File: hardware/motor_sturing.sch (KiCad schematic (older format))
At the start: 6 parts, among them U1 LTC2351-14, U22 LTC2351-14, U5 MAX6101

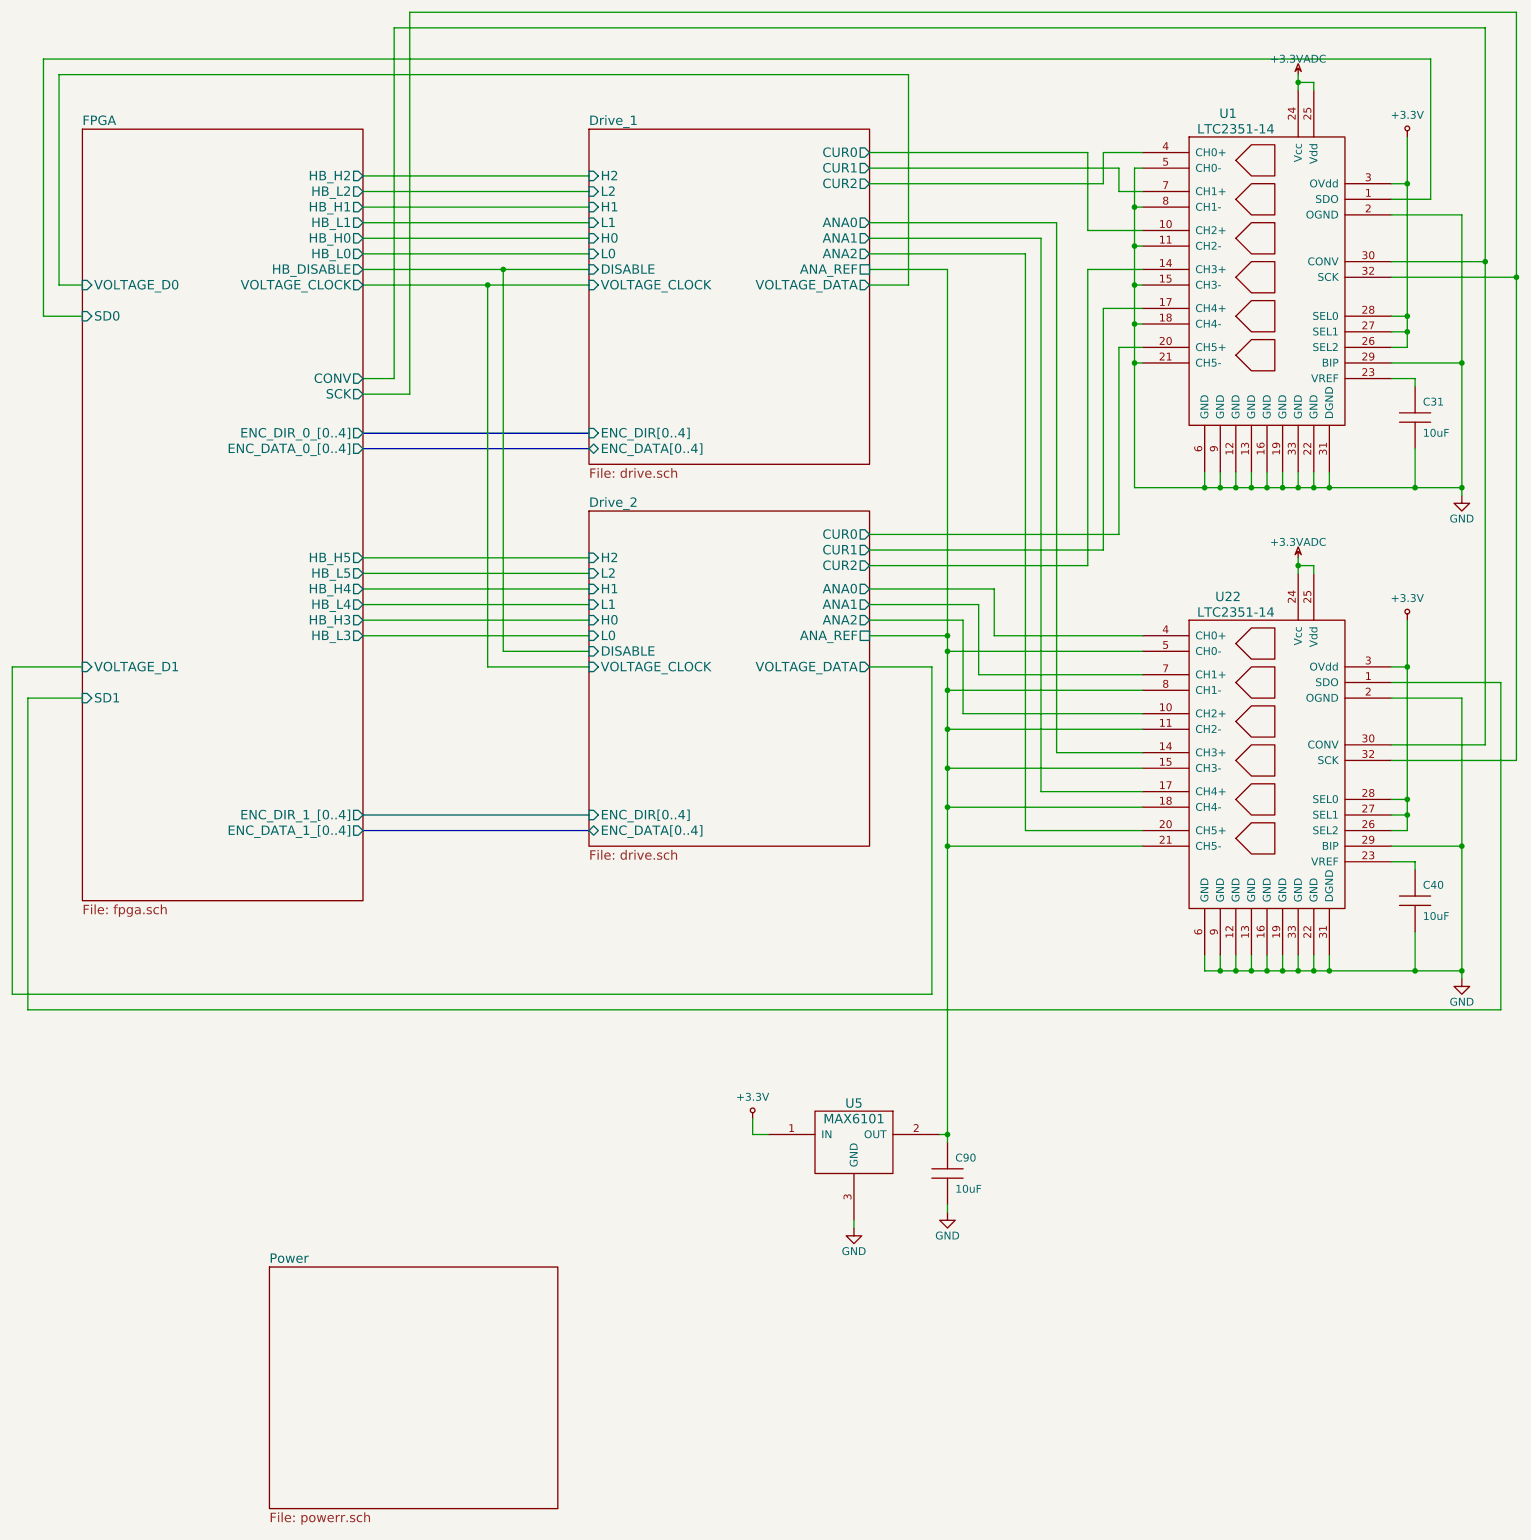
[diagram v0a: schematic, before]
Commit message: Progress.
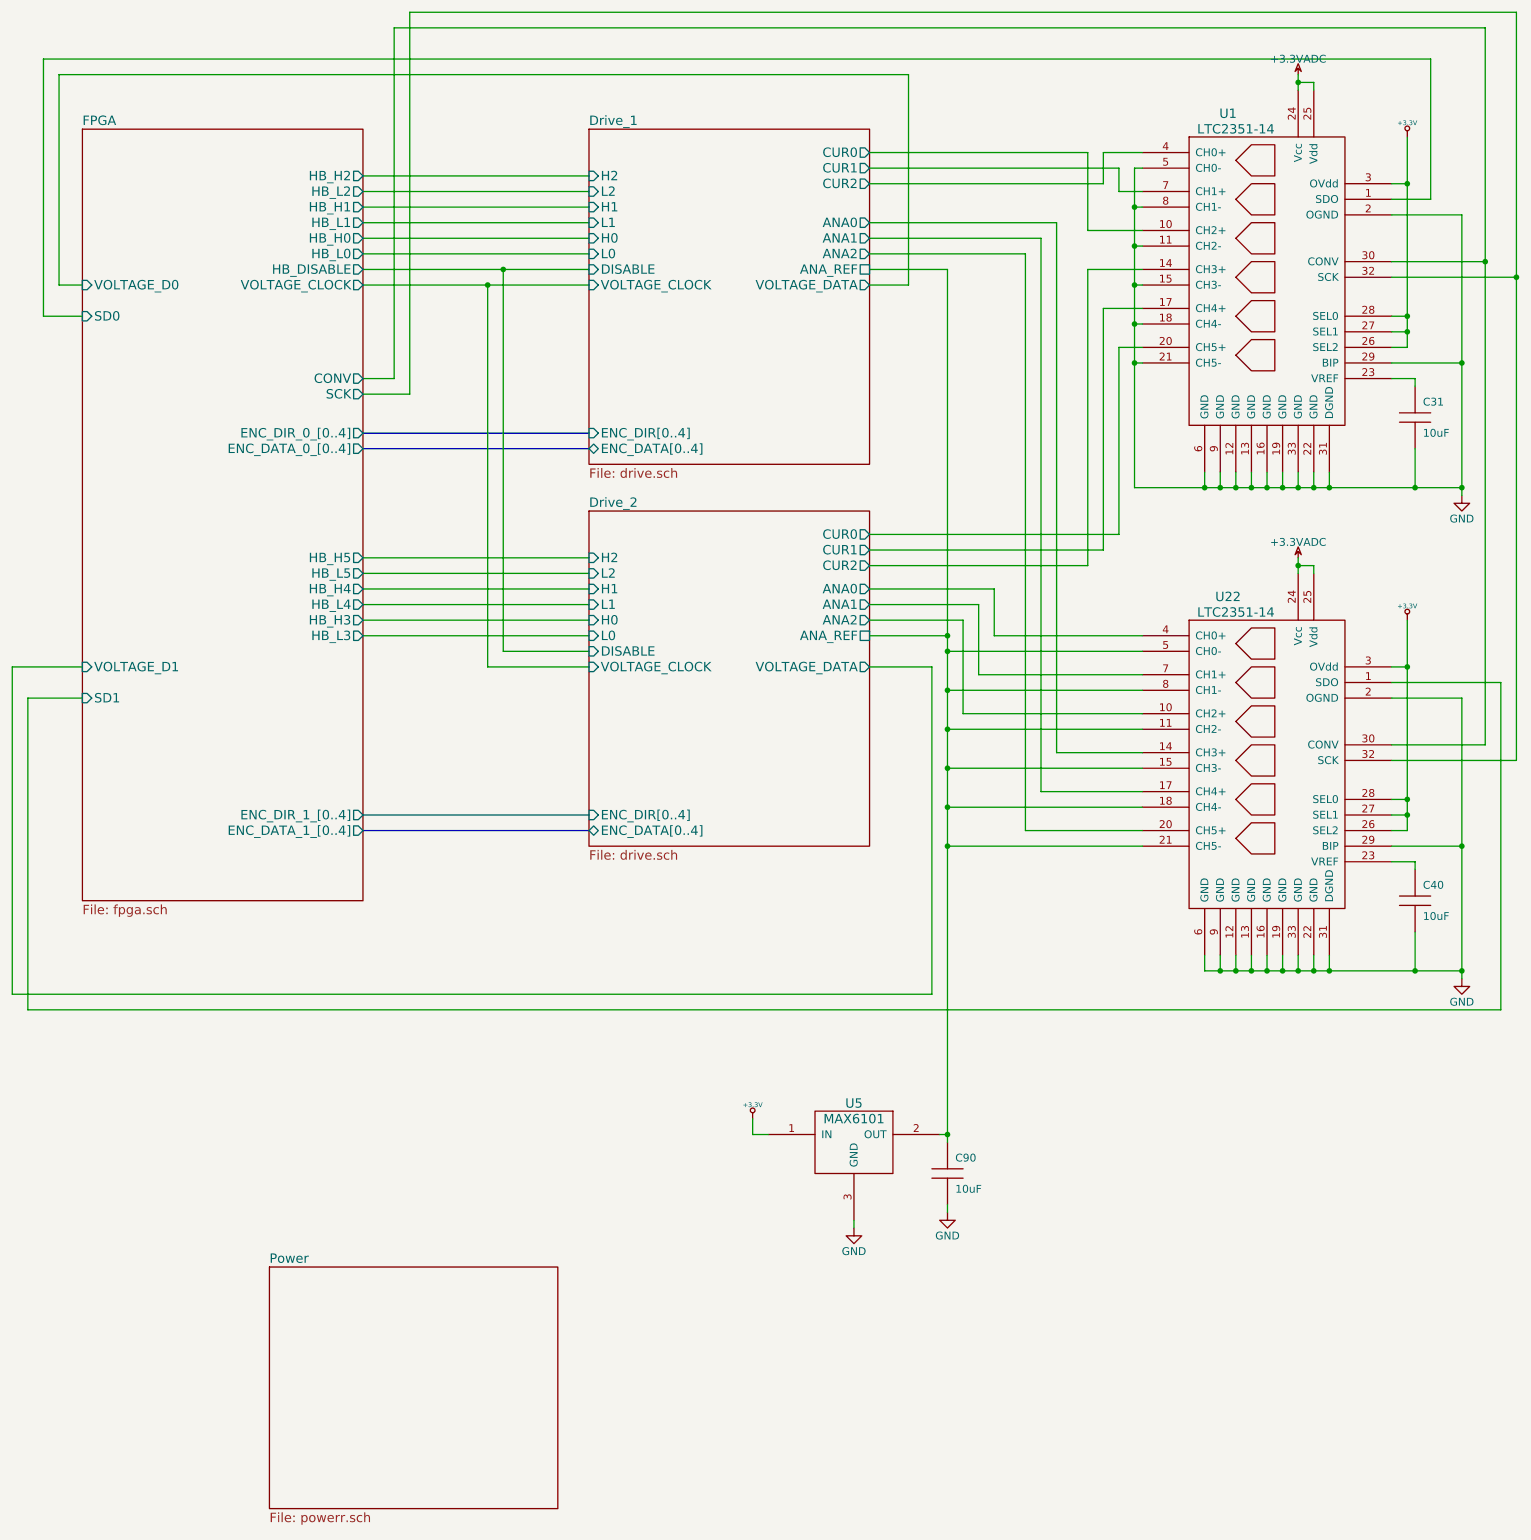
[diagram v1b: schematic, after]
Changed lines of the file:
@@
 Connection ~ 8500 1850
 $Comp
-L +3.3VADC #PWR198
+L +3.3VADC #PWR218
 U 1 1 56D0AB8B
 P 9550 4100
-F 0 "#PWR198" H 9700 4050 50  0001 C CNN
+F 0 "#PWR218" H 9700 4050 50  0001 C CNN
 F 1 "+3.3VADC" H 9550 4200 50  0000 C CNN
 F 2 "" H 9550 4100 50  0000 C CNN
@@
 	9650 4150 9650 4200
 Connection ~ 9550 4150
-$Comp
-L +3.3V #PWR199
-U 1 1 56D0BAED
-P 10250 1400
-F 0 "#PWR199" H 10250 1250 50  0001 C CNN
-F 1 "+3.3V" H 10250 1540 50  0000 C CNN
-F 2 "" H 10250 1400 50  0000 C CNN
-F 3 "" H 10250 1400 50  0000 C CNN
-	1    10250 1400
-	1    0    0    -1
-$EndComp
 Wire Wire Line
 	10250 1400 10250 2750
@@
 	10250 1700 10150 1700
 $Comp
-L GND #PWR201
+L GND #PWR221
 U 1 1 56D0BF5F
 P 10600 3700
-F 0 "#PWR201" H 10600 3450 50  0001 C CNN
+F 0 "#PWR221" H 10600 3450 50  0001 C CNN
 F 1 "GND" H 10600 3550 50  0000 C CNN
 F 2 "" H 10600 3700 50  0000 C CNN
@@
 	1    0    0    -1
 $EndComp
-$Comp
-L +3.3V #PWR200
-U 1 1 56D10ACF
-P 10250 4500
-F 0 "#PWR200" H 10250 4350 50  0001 C CNN
-F 1 "+3.3V" H 10250 4640 50  0000 C CNN
-F 2 "" H 10250 4500 50  0000 C CNN
-F 3 "" H 10250 4500 50  0000 C CNN
-	1    10250 4500
-	1    0    0    -1
-$EndComp
 Wire Wire Line
 	10250 4500 10250 5850
@@
 	10250 4800 10150 4800
 $Comp
-L GND #PWR202
+L GND #PWR222
 U 1 1 56D10AD7
 P 10600 6800
-F 0 "#PWR202" H 10600 6550 50  0001 C CNN
+F 0 "#PWR222" H 10600 6550 50  0001 C CNN
 F 1 "GND" H 10600 6650 50  0000 C CNN
 F 2 "" H 10600 6800 50  0000 C CNN
@@
 	1    0    0    -1
 $EndComp
-$Comp
-L +3.3V #PWR194
-U 1 1 56D1582B
-P 6050 7700
-F 0 "#PWR194" H 6050 7550 50  0001 C CNN
-F 1 "+3.3V" H 6050 7840 50  0000 C CNN
-F 2 "" H 6050 7700 50  0000 C CNN
-F 3 "" H 6050 7700 50  0000 C CNN
-	1    6050 7700
-	1    0    0    -1
-$EndComp
 Wire Wire Line
 	6050 7700 6050 7800
@@
 	6050 7800 6150 7800
 $Comp
-L GND #PWR195
+L GND #PWR215
 U 1 1 56D15D96
 P 6700 8400
-F 0 "#PWR195" H 6700 8150 50  0001 C CNN
+F 0 "#PWR215" H 6700 8150 50  0001 C CNN
 F 1 "GND" H 6700 8250 50  0000 C CNN
 F 2 "" H 6700 8400 50  0000 C CNN
@@
 Connection ~ 10950 2300
 $Comp
-L +3.3VADC #PWR197
+L +3.3VADC #PWR217
 U 1 1 56D1B9BD
 P 9550 1000
-F 0 "#PWR197" H 9700 950 50  0001 C CNN
+F 0 "#PWR217" H 9700 950 50  0001 C CNN
 F 1 "+3.3VADC" H 9550 1100 50  0000 C CNN
 F 2 "" H 9550 1000 50  0000 C CNN
@@
 Connection ~ 7300 7800
 $Comp
-L GND #PWR196
+L GND #PWR216
 U 1 1 56D58C47
 P 7300 8300
-F 0 "#PWR196" H 7300 8050 50  0001 C CNN
+F 0 "#PWR216" H 7300 8050 50  0001 C CNN
 F 1 "GND" H 7300 8150 50  0000 C CNN
 F 2 "" H 7300 8300 50  0000 C CNN
@@
 Wire Wire Line
 	8200 4150 6800 4150
+$Comp
+L +3.3V #PWR214
+U 1 1 56DB5355
+P 6050 7700
+F 0 "#PWR214" H 6100 7730 20  0001 C CNN
+F 1 "+3.3V" H 6050 7790 30  0000 C CNN
+F 2 "" H 6050 7700 60  0000 C CNN
+F 3 "" H 6050 7700 60  0000 C CNN
+	1    6050 7700
+	1    0    0    -1
+$EndComp
+$Comp
+L +3.3V #PWR219
+U 1 1 56DBFBBB
+P 10250 1400
+F 0 "#PWR219" H 10300 1430 20  0001 C CNN
+F 1 "+3.3V" H 10250 1490 30  0000 C CNN
+F 2 "" H 10250 1400 60  0000 C CNN
+F 3 "" H 10250 1400 60  0000 C CNN
+	1    10250 1400
+	1    0    0    -1
+$EndComp
+$Comp
+L +3.3V #PWR220
+U 1 1 56DC019F
+P 10250 4500
+F 0 "#PWR220" H 10300 4530 20  0001 C CNN
+F 1 "+3.3V" H 10250 4590 30  0000 C CNN
+F 2 "" H 10250 4500 60  0000 C CNN
+F 3 "" H 10250 4500 60  0000 C CNN
+	1    10250 4500
+	1    0    0    -1
+$EndComp
 $EndSCHEMATC
